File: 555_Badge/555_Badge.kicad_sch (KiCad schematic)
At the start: 15 parts, among them Q1 2N3904

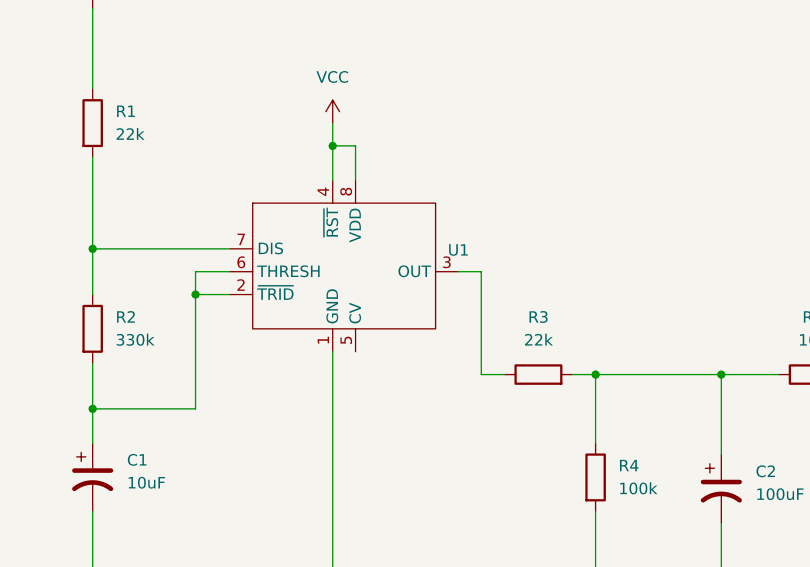
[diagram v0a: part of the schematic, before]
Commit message: update schema
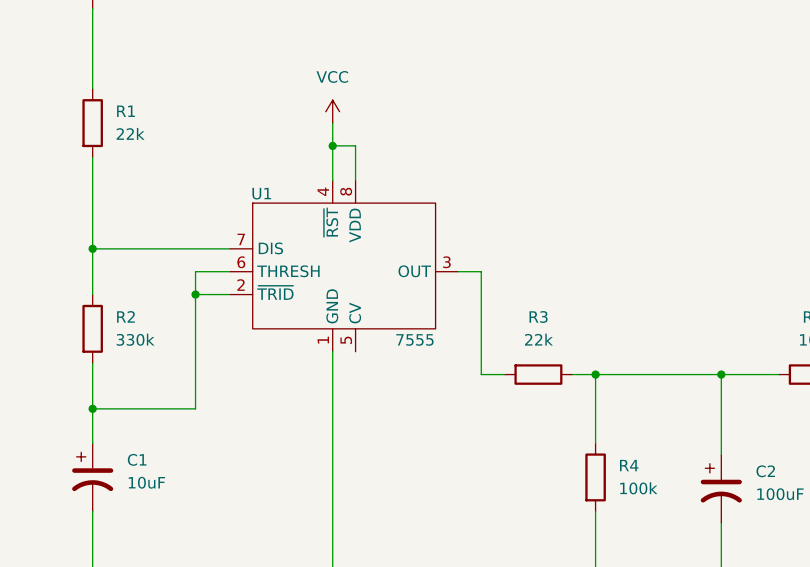
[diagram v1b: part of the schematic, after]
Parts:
- C1: footprint (none) -> Capacitor_THT:CP_Radial_D5.0mm_P2.00mm
- C2: footprint (none) -> Capacitor_THT:CP_Radial_D6.3mm_P2.50mm
- D1, D2: footprint (none) -> LED_THT:LED_D3.0mm
- Q1: footprint Package_TO_SOT_THT:TO-92_Inline -> digikey-footprints:TO-92-3
- R1, R2, R3, R4, R5, R6, R7: footprint (none) -> Resistor_THT:R_Axial_DIN0207_L6.3mm_D2.5mm_P7.62mm_Horizontal
- U1: value ~ -> 7555; footprint (none) -> 555_Badge:ICM7555-PDIP
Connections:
- net at U1.3 (OUT): now also R3.2; no longer R3.1
- net at C2.1, R4.1, R5.1: now also R3.1; no longer R3.2
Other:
- moved on the sheet: R3
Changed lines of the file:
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@@
 			)
 		)
-		(property "Footprint" ""
+		(property "Footprint" "Capacitor_THT:CP_Radial_D5.0mm_P2.00mm"
 			(at 95.25 134.62 0)
 			(effects
@@
 			)
 		)
-		(property "Footprint" ""
+		(property "Footprint" "LED_THT:LED_D3.0mm"
 			(at 194.31 101.6 0)
 			(effects
@@
 		(on_board yes)
 		(dnp no)
-		(fields_autoplaced yes)
 		(property "Reference" "U1"
-			(at 135.89 109.382 0)
-			(effects
-				(font
-					(size 1.27 1.27)
-				)
-			)
-		)
-		(property "Value" "~"
-			(at 135.89 111.2871 0)
-			(effects
-				(font
-					(size 1.27 1.27)
-				)
-			)
-		)
-		(property "Footprint" ""
+			(at 114.046 103.124 0)
+			(effects
+				(font
+					(size 1.27 1.27)
+				)
+			)
+		)
+		(property "Value" "7555"
+			(at 131.064 119.38 0)
+			(effects
+				(font
+					(size 1.27 1.27)
+				)
+			)
+		)
+		(property "Footprint" "555_Badge:ICM7555-PDIP"
 			(at 123.19 109.22 0)
 			(effects
@@
 			)
 		)
-		(property "Footprint" ""
+		(property "Footprint" "Resistor_THT:R_Axial_DIN0207_L6.3mm_D2.5mm_P7.62mm_Horizontal"
 			(at 209.042 87.63 90)
 			(effects
@@
 			)
 		)
-		(property "Footprint" ""
+		(property "Footprint" "Capacitor_THT:CP_Radial_D6.3mm_P2.50mm"
 			(at 165.1 135.89 0)
 			(effects
@@
 			)
 		)
-		(property "Footprint" ""
+		(property "Footprint" "Resistor_THT:R_Axial_DIN0207_L6.3mm_D2.5mm_P7.62mm_Horizontal"
 			(at 93.472 118.11 90)
 			(effects
@@
 			)
 		)
-		(property "Footprint" ""
+		(property "Footprint" "Resistor_THT:R_Axial_DIN0207_L6.3mm_D2.5mm_P7.62mm_Horizontal"
 			(at 149.352 134.62 90)
 			(effects
@@
 			)
 		)
-		(property "Footprint" ""
+		(property "Footprint" "LED_THT:LED_D3.0mm"
 			(at 210.82 101.6 0)
 			(effects
@@
 			)
 		)
-		(property "Footprint" ""
+		(property "Footprint" "Resistor_THT:R_Axial_DIN0207_L6.3mm_D2.5mm_P7.62mm_Horizontal"
 			(at 192.532 87.63 90)
 			(effects
@@
 			)
 		)
-		(property "Footprint" ""
+		(property "Footprint" "Resistor_THT:R_Axial_DIN0207_L6.3mm_D2.5mm_P7.62mm_Horizontal"
 			(at 93.472 95.25 90)
 			(effects
@@
 			)
 		)
-		(property "Footprint" "Package_TO_SOT_THT:TO-92_Inline"
+		(property "Footprint" "digikey-footprints:TO-92-3"
 			(at 196.85 125.095 0)
 			(effects
@@
 			)
 		)
-		(property "Footprint" ""
+		(property "Footprint" "Resistor_THT:R_Axial_DIN0207_L6.3mm_D2.5mm_P7.62mm_Horizontal"
 			(at 175.26 124.968 90)
 			(effects
@@
 	(symbol
 		(lib_id "Device:R")
-		(at 144.78 123.19 90)
+		(at 144.78 123.19 270)
 		(unit 1)
 		(exclude_from_sim no)
@@
 			)
 		)
-		(property "Footprint" ""
-			(at 144.78 124.968 90)
-			(effects
-				(font
+		(property "Footprint" "Resistor_THT:R_Axial_DIN0207_L6.3mm_D2.5mm_P7.62mm_Horizontal"
+			(at 144.78 121.412 90)
+			(effects
+				(font
